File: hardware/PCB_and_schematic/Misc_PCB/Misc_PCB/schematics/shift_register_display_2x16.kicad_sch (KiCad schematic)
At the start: 15 parts, among them J4 LCD_CONN, J6 LCD_DISPLAY, Q8 BC547, U4 74HC595

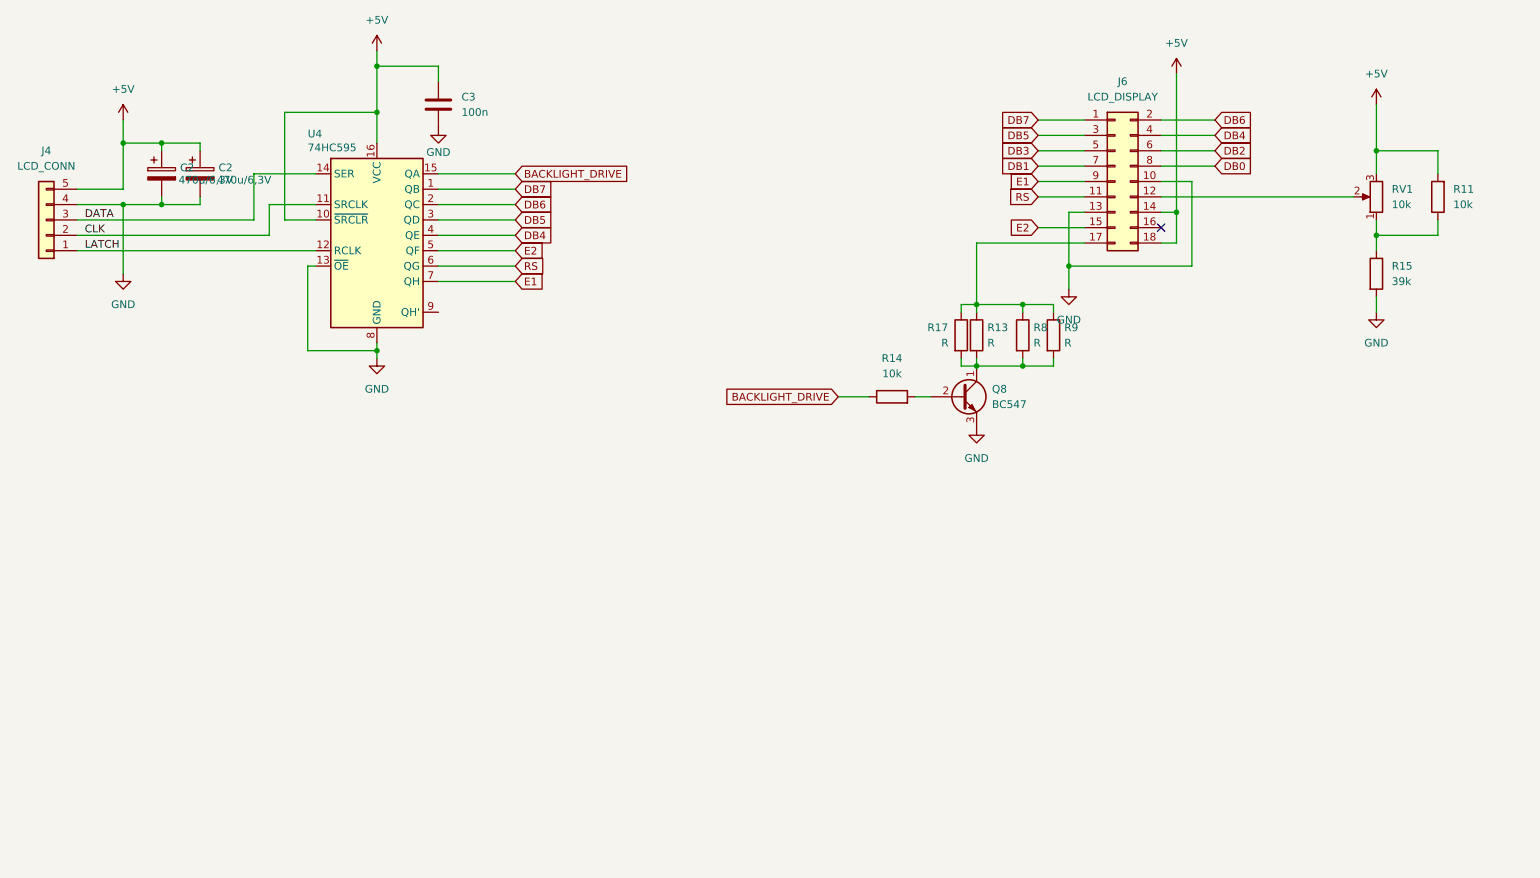
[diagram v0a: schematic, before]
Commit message: progress with esp power pcb
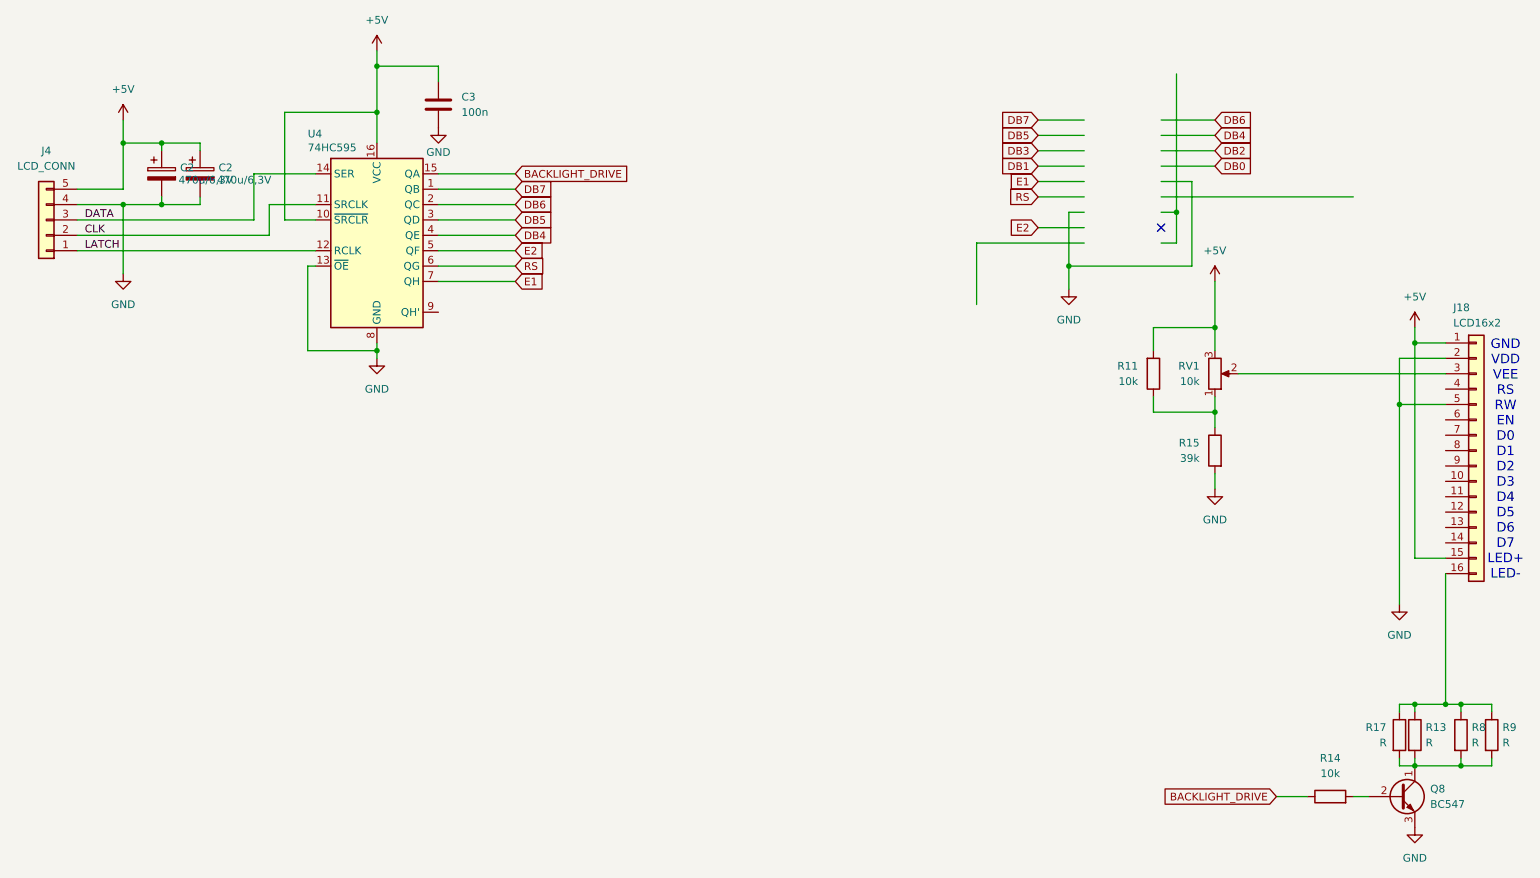
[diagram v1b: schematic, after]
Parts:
- removed J6: LCD_DISPLAY, Connector_PinHeader_2.54mm:PinHeader_2x09_P2.54mm_Vertical, symbol Connector_Generic:Conn_02x09_Odd_Even
- added J18: LCD16x2, symbol Connector_Generic:Conn_01x16
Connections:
- net +5V: now also J18.1 (Pin_1), J18.15 (Pin_15)
- net GND: now also J18.2 (Pin_2), J18.5 (Pin_5)
- net at R13.1, R17.1, R8.1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: now also J18.16 (Pin_16)
- net at RV1.2: now also J18.3 (Pin_3)
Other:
- note added: "GND VDD VEE RS RW EN D0 D1 D2 D3 D4 D5 D6 D7 LED+ LED-"
- moved on the sheet: Q8, R11, R13, R14, R15, R17, R8, R9, RV1
